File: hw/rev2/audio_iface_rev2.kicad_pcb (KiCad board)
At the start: 4 copper layers, 66 x 24.8 mm, 151 parts, among them J1 COAX, J2 CONN_01X02, J3 USBMICROCONN, J4 CONN_01X02, J5 CONN_01X02, J6 COAX, J7 COAX, J9 CONN_01X02, P3 CONN_01X06, U1 LT6241, U2 LTC6242, U3 AK4621, U4 K20X7_QFP64, U5 TPS61252, U6 LP2992AILD-5.0, U7 LTC6242, U8 TPA6130A2, U9 MT29FXX01A, X1 XTAL, X2 ASFLM2-12.288MHZ

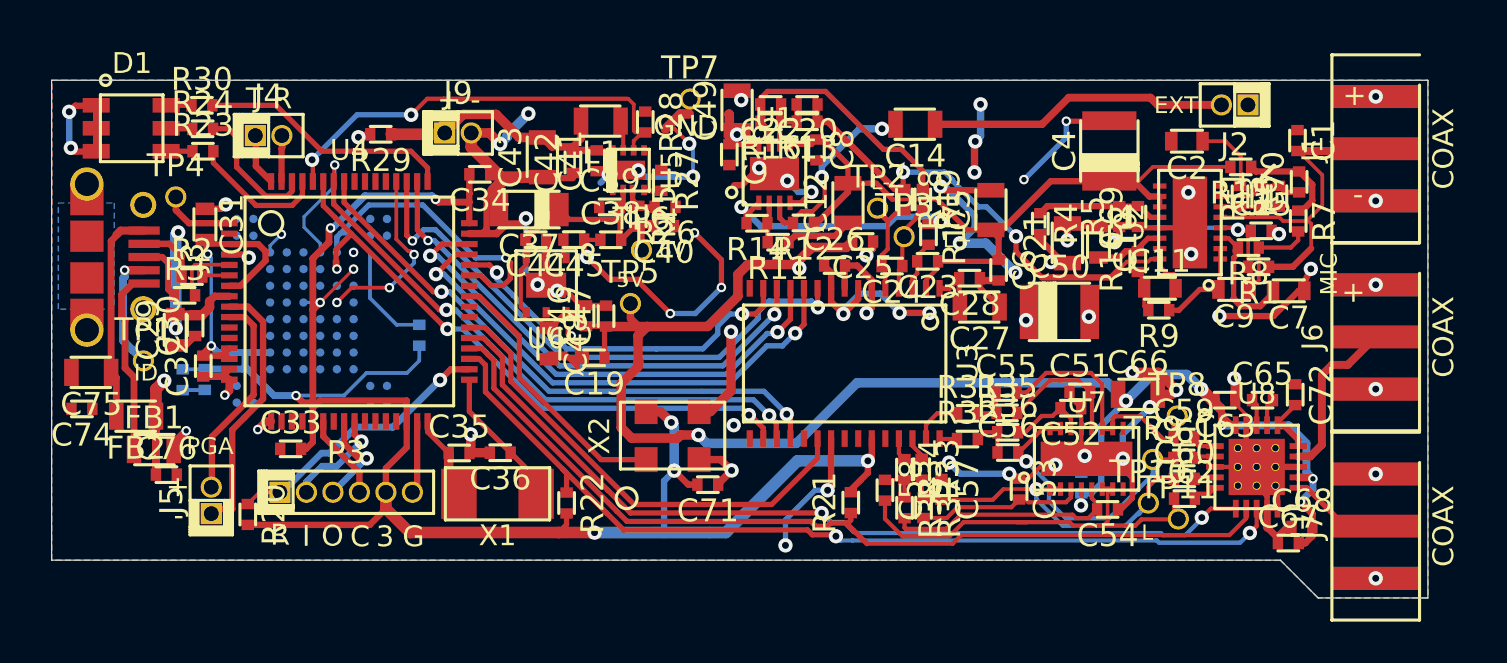
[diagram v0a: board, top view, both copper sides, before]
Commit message: More routing
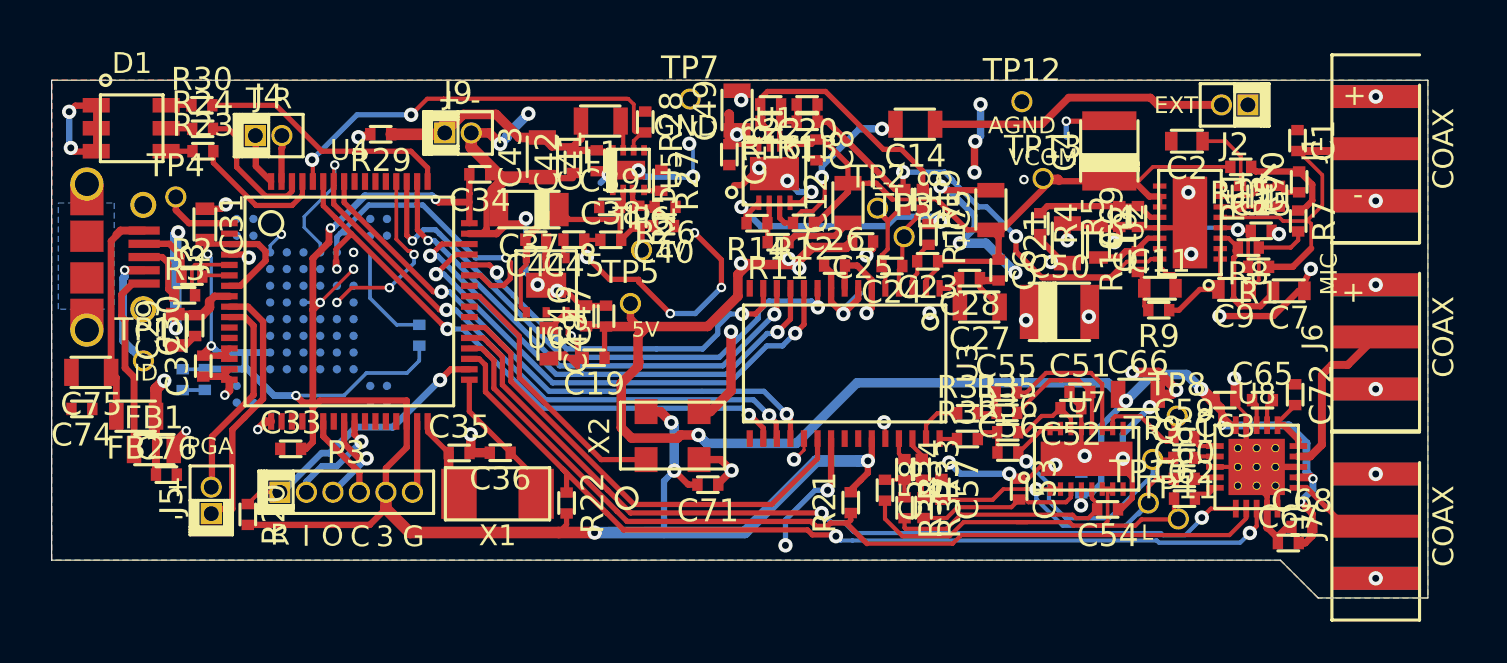
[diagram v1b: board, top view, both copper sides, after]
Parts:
- added TP12: TP, lib:TP_HOLE, F.Cu at (198.5, 73.0)
- added TP13: TP, lib:TP_HOLE, F.Cu at (199.5, 76.7)
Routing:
- net AGND_IN: track 199.1 -> 195.0 mm, vias 63 -> 62
- net +5VA: track 124.4 -> 125.5 mm, vias 13 -> 15
- net VCOM_VRT: track 36.9 -> 37.8 mm
- net (no net): track 3.38 -> 3.49 mm, vias 4 -> 5
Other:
- board text added: "AGND"
- board text added: "VCOM"
